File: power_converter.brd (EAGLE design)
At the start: 49.5 x 49.5 mm, 20 parts

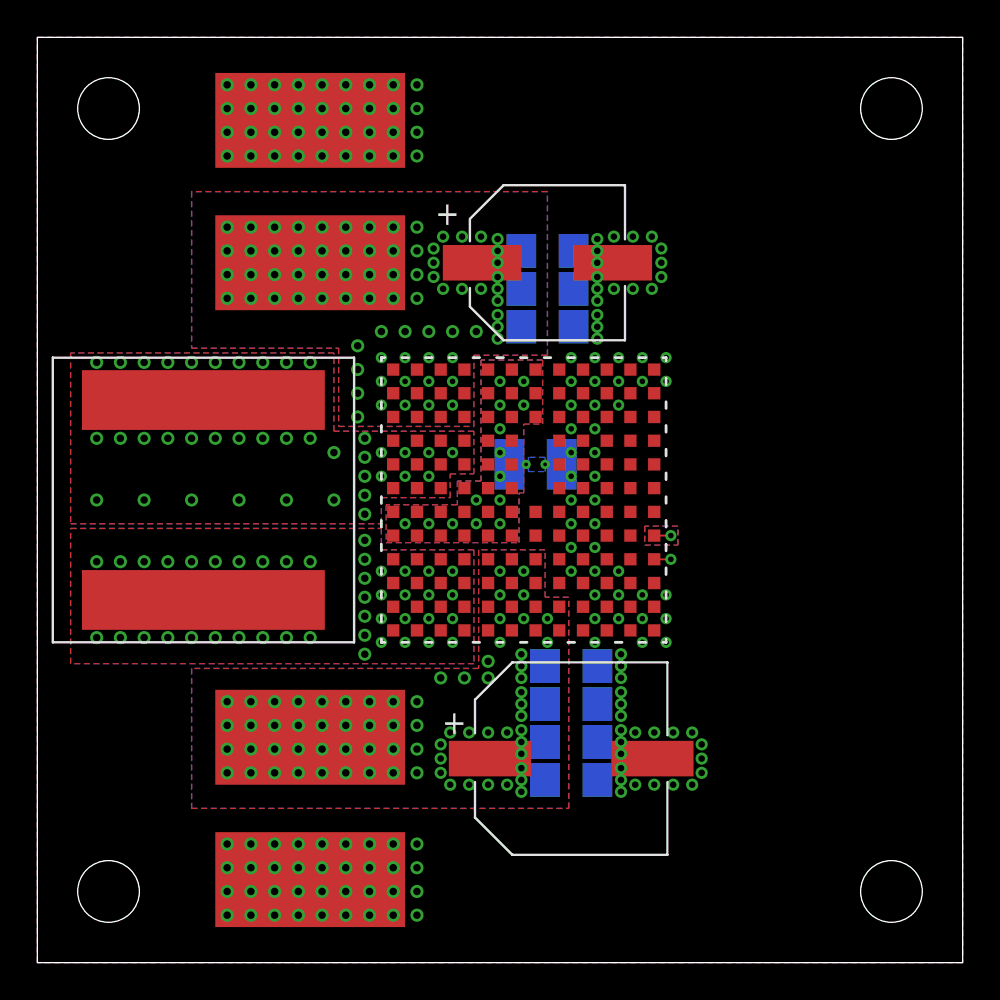
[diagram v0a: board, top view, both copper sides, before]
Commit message: Completed revision 1.0
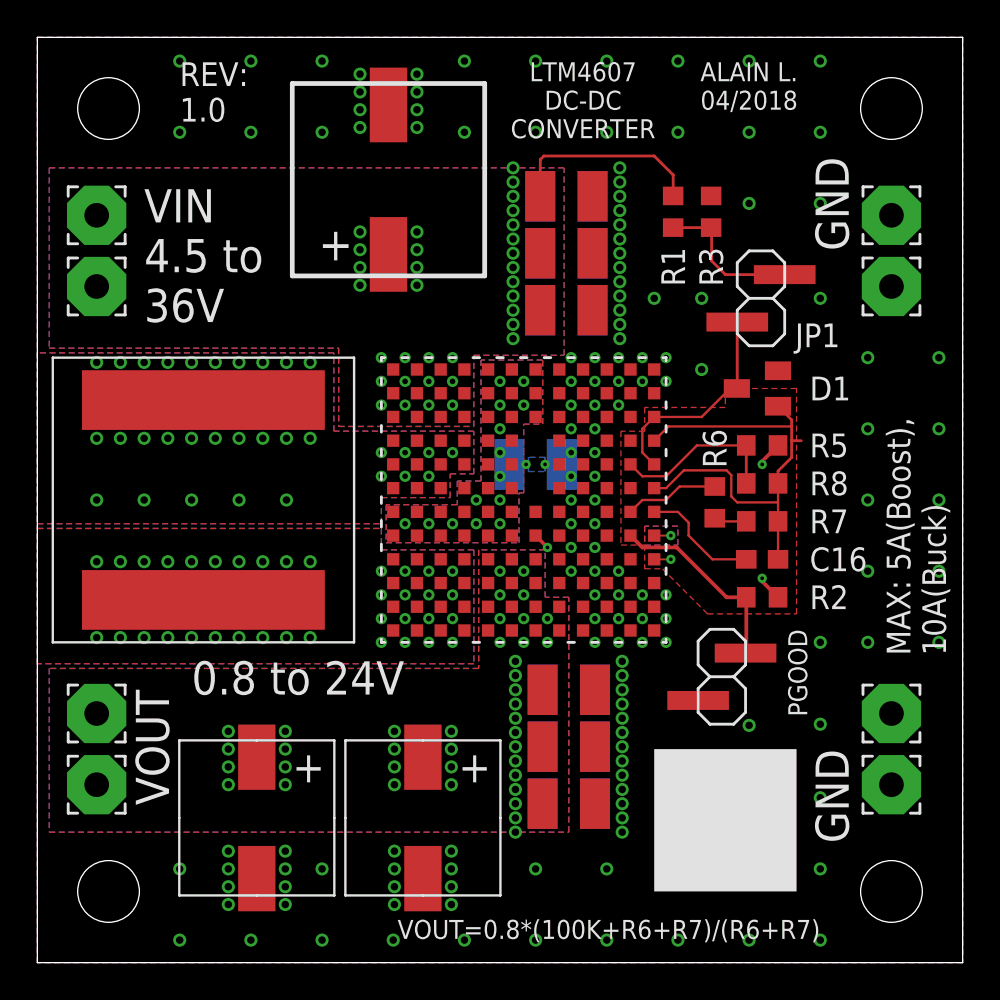
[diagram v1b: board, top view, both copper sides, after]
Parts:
- added C10, C11, C12, C13: 10u, rcl:C1210
- added C14, C15: 220u, LTM4607:PCR1V221MCL1GS
- added C16: 5n, rcl:C0603
- added D1: 4.7V, LTM4607:SOT23
- added JP1, JP2: (no value), pinhead-2:1X02SMD
- added PAD5, PAD6, PAD7, PAD8: (no value), wirepad:3,17/1,3
- added R2: 100k, rcl:R0603
- added R3: 8.5k, rcl:R0603
- added R4: 7m, rcl:R1210
- added R5: 4.7k, rcl:R0603
- added R6: 150, rcl:R0603
- added R7: 6.98k, rcl:R0603
- added R8: 2.7k, rcl:R0603
- added U$5: (no value), frames:A4L-LOC
- C1, C2, C3, C5, C8, C9: value (none) -> 10u; device rcl:C1206 -> rcl:C1210
- C4: value (none) -> 10u; device Kondensatoren (rev17a):4.4X1.9X4.3(BXCXA) -> rcl:C1210
- C6: value (none) -> 10u; device Kondensatoren (rev17a):4.2X1.9X2.8(BXCXA) -> rcl:C1210
- C7: value (none) -> 180u; device rcl:C1206 -> LTM4607:PCR1H181MCL1GS
- L1: value (none) -> 4.7u
- PAD1, PAD2, PAD3, PAD4: device LTM4607:SMD5,08-10,16 -> wirepad:3,17/1,3
- R1: value (none) -> 51k; device rcl:R1210 -> rcl:R0603
- moved PAD2 37.4 mm to (3.17, 40.0), turned to 0 degrees
- moved PAD4 37.4 mm to (3.17, 9.53), turned to 0 degrees
- moved PAD1 26.7 mm to (3.17, 36.2)
- moved PAD3 26.7 mm to (3.17, 13.3)
- moved C9 26.6 mm to (28.4, 11.6)
- moved C3 26.2 mm to (28.3, 38.0), flipped to the top, turned to 0 degrees
- moved C4 24.0 mm to (28.3, 34.9), turned to 0 degrees
- moved C1 22.1 mm to (28.3, 38.0)
- moved C2 21.1 mm to (28.3, 34.9)
- moved R1 15.4 mm to (34.0, 40.2), flipped to the top, turned to 90 degrees
- moved C7 10.3 mm to (18.8, 41.9), flipped to the top
- moved C5 7.06 mm to (28.3, 41.0)
- moved C8 4.83 mm to (28.4, 14.6), flipped to the top, turned to 0 degrees
- moved C6 3.70 mm to (28.3, 41.0), turned to 0 degrees
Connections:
- removed net FCB: U1.A9
- removed net STBMD: U1.A10
- new net N$1: R6.1, R7.2
- new net N$2: JP1.2, R1.1, R3.2
- net GND: now also C10.2, C11.2, C12.2, C13.2, C14.NEG, C15.NEG, C16.1, C7.NEG, D1.1, JP2.2, PAD5.1, PAD6.1, PAD7.1, PAD8.1, R3.1, R4.2, R7.1, R8.2, U1.A9; no longer C7.2, PAD2.1, PAD4.1, R1.2
- net INTVCC: now also R2.1, R5.2
- net PGOOD: now also JP2.1, R2.2
- net PLLFLTR: now also R5.1, R8.1
- net RSENSE: now also R4.1; no longer R1.1
- net RUN: now also D1.3, JP1.1, U1.A10
- net SS: now also C16.2
- net VFB: now also R6.2
- net VIN: now also C1.1, C2.1, C3.1, C4.1, C7.POS, PAD1.1, PAD2.1, R1.2; no longer C7.1, C9.1, PAD3.1
- net VOUT: now also C10.1, C11.1, C12.1, C13.1, C14.POS, C15.POS, C9.1, PAD3.1, PAD4.1; no longer C1.1, C2.1, C3.1, C4.1, PAD1.1
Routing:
- net GND: track 12.4 -> 37.8 mm, vias 154 -> 149
- net INTVCC: track 0.00 -> 22.6 mm, vias 0 -> 3
- net RUN: track 0.00 -> 11.8 mm
- net VIN: track 0.00 -> 10.7 mm, vias 75 -> 33
- net PGOOD: track 0.00 -> 10.7 mm
- net PLLFLTR: track 0.00 -> 9.18 mm
- net N$2: track 0.00 -> 8.09 mm
- net SS: track 0.00 -> 6.39 mm
- net VFB: track 0.00 -> 5.07 mm
- net N$1: track 0.00 -> 1.76 mm
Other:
- board text added: "0.8 to 24V"
- board text added: "4 layer design"
- board text added: "ALAIN L. 04/2018"
- board text added: "Filled silk-screen square to be used for noting designed output voltage"
- board text added: "GND"
- board text added: "LTM4607 DC-DC CONVERTER"
- board text added: "MAX: 5A(Boost), 10A(Buck)"
- board text added: "Mounting holes sized for 4-40 screws"
- board text added: "PGOOD"
- board text added: "REV: 1.0"
- board text added: "Stencil and reflow soldering are highly recommended for this design"
- board text added: "Through-hole wirepads sized for 18AWG wire"
- board text added: "VIN 4.5 to 36V"
- board text added: "VOUT"
- board text added: "VOUT=0.8*(100K+R6+R7)/(R6+R7)"
